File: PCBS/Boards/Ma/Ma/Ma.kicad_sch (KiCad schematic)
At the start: 39 parts, among them J1 Conn_01x02_Socket, J10 Conn_01x14_Pin, J2 Conn_01x04_Socket, J3 Conn_01x02_Pin, J4 Conn_01x02_Pin, J5 Conn_01x03_Pin, J7 Conn_01x03_Pin, J8 Conn_01x06_Socket, J9 Conn_01x04_Socket, SW1 SW_Push, SW2 SW_SPDT, SW3 SW_Push, SW4 SW_Push, U1 ATmega328P-M, Y1 Crystal

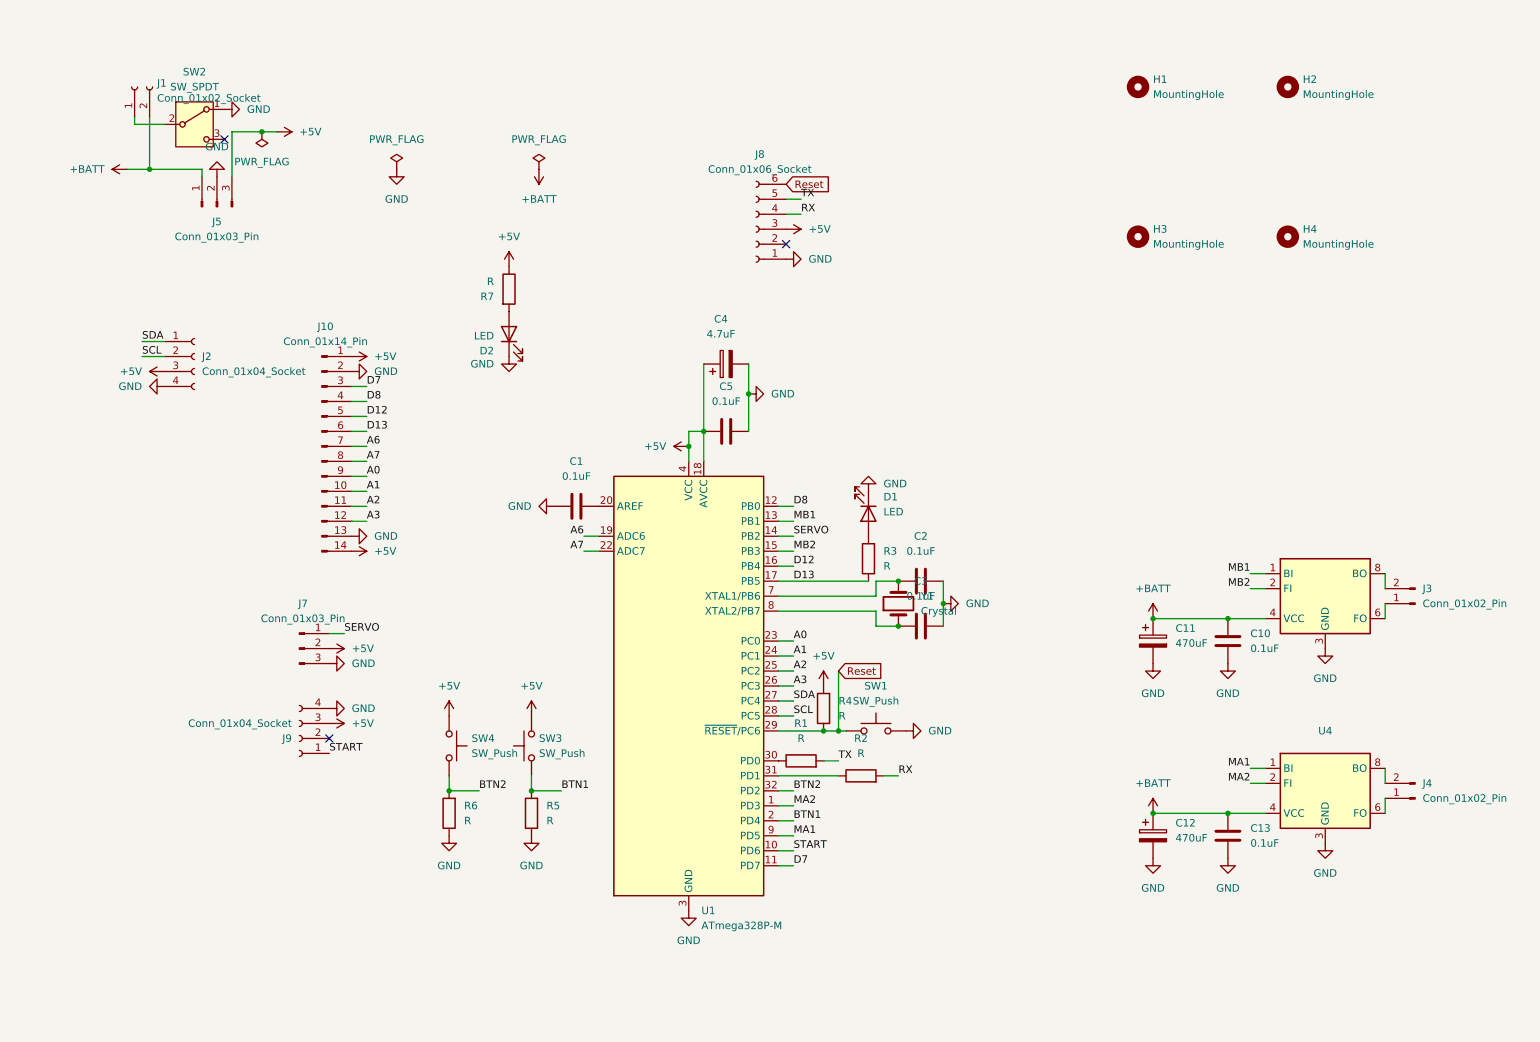
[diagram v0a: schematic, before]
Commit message: updated readme and PCB files
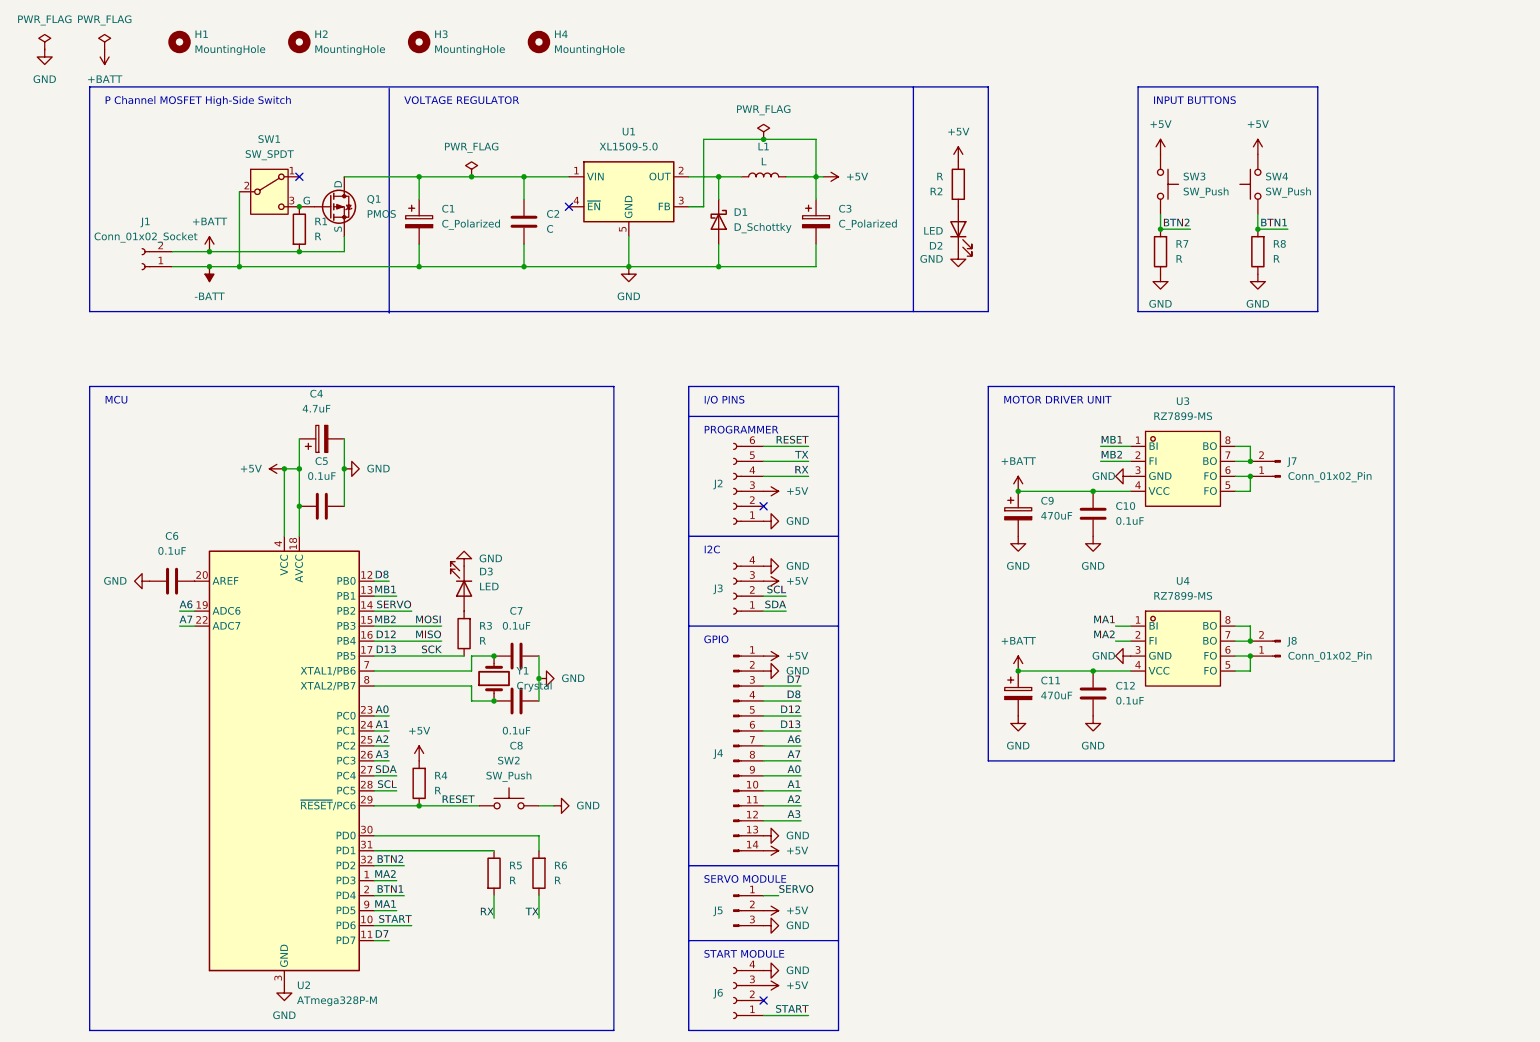
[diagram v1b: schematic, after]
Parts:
- removed J2, J9: Conn_01x04_Socket, Connector_PinSocket_2.54mm:PinSocket_1x04_P2.54mm_Vertical, symbol Connector:Conn_01x04_Socket
- removed J5: Conn_01x03_Pin, Package_TO_SOT_SMD:TO-252-2, symbol Connector:Conn_01x03_Pin
- removed U3, U4: ~, Package_SO:SOP-8_3.9x4.9mm_P1.27mm, symbol Custom Development Boards:RZ7899_1
- added C1, C3: C_Polarized, symbol Device:C_Polarized
- added C2: C, symbol Device:C
- added D1: D_Schottky, symbol Device:D_Schottky
- added J3, J6: Conn_01x04_Socket, symbol Connector:Conn_01x04_Socket
- added L1: L, symbol Device:L
- added Q1: PMOS, symbol Simulation_SPICE:PMOS
- added R1: R, symbol Device:R
- added U1: XL1509-5.0, Package_SO:SOIC-8_3.9x4.9mm_P1.27mm, symbol Regulator_Switching:XL1509-5.0
- added U3, U4: RZ7899-MS, EasyEDA:SOIC-8_L4.9-W3.9-P1.27-LS6.0-BL, symbol EasyEDA:RZ7899-MS
- renumbered C12 to C11, C13 to C12, C1 to C6, C2 to C7, C3 to C8, C11 to C9, D1 to D3, J8 to J2, J10 to J4, J7 to J5, J3 to J7, J4 to J8, R7 to R2, R2 to R5, R1 to R6, R6 to R7, R5 to R8, SW2 to SW1, SW1 to SW2, SW4 to SW3, SW3 to SW4, U1 to U2
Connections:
- net +5V: now also C3.1, J3.3 (Pin_3), J6.3 (Pin_3), L1.2, U1.3 (FB)
- net +BATT: now also Q1.3 (S), R1.2, U3.4 (VCC), U4.4 (VCC)
- net MA1: now also U4.1 (BI)
- net MA2: now also U4.2 (FI)
- net MB1: now also U3.1 (BI)
- net MB2: now also U3.2 (FI)
- net SCL: now also J3.2 (Pin_2)
- net SDA: now also J3.1 (Pin_1)
- net START: now also J6.1 (Pin_1)
- net TX: now also R6.1; no longer R6.2
- net -BATT: now reaches J1.1 (Pin_1), SW1.2 (B)
- net -BATT: now also C10.2, C11.2, C12.2, C4.2, C5.2, C6.1, C7.2, C8.2, C9.2, D2.1 (K), D3.1 (K), J2.1 (Pin_1), J4.13 (Pin_13), J4.2 (Pin_2), J5.3 (Pin_3), R7.1, R8.1, SW2.2, U2.21 (GND), U2.3 (GND), U2.33 (GND), U2.5 (GND), C1.2, C2.2, C3.2, D1.2 (A), J3.4 (Pin_4), J6.4 (Pin_4), U1.5 (GND), U1.6 (GND), U1.7 (GND), U1.8 (GND), U3.3 (GND), U4.3 (GND)
- net at SW1.3 (C): now also Q1.2 (G), R1.1
- net at J8.1 (Pin_1): now also U4.5 (FO), U4.6 (FO)
- net at J8.2 (Pin_2): now also U4.7 (BO), U4.8 (BO)
- net at U2.30 (PD0): now also R6.2; no longer R6.1
- net at J7.1 (Pin_1): now also U3.5 (FO), U3.6 (FO)
- net at J7.2 (Pin_2): now also U3.7 (BO), U3.8 (BO)
- removed net GND: C10.2, C11.2, C12.2, C4.2, C5.2, C6.1, C7.2, C8.2, C9.2, D2.1 (K), D3.1 (K), J2.1 (Pin_1), J4.13 (Pin_13), J4.2 (Pin_2), J5.3 (Pin_3), R7.1, R8.1, SW1.1 (A), SW2.2, U2.21 (GND), U2.3 (GND), U2.33 (GND), U2.5 (GND)
- net Reset renamed RESET
- new net: C1.1, C2.1, Q1.1 (D), U1.1 (VIN)
- new net: D1.1 (K), L1.1, U1.2 (OUT)
- no-connect marks 3 -> 4
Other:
- note added: "GPIO"
- note added: "I/O PINS"
- note added: "I2C"
- note added: "INPUT BUTTONS"
- note added: "MCU"
- note added: "MOTOR DRIVER UNIT"
- note added: "P Channel MOSFET High-Side Switch"
- note added: "PROGRAMMER"
- note added: "SERVO MODULE"
- note added: "START MODULE"
- note added: "VOLTAGE REGULATOR"
- company: (none) -> DENJU DIVISION
- title: (none) -> Ma AIO Board
- moved on the sheet: C10, C11, C12, C4, C5, C6, C7, C8, C9, D2, D3, H1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
